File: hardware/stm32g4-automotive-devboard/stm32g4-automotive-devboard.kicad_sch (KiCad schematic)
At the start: 0 parts

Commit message: Added mcu and trancievers to sch
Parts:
- added U1: STM32G431CBTx, Package_QFP:LQFP-48_7x7mm_P0.5mm, symbol MCU_ST_STM32G4:STM32G431CBTx
- added U2, U3: TJA1051T-3, Package_SO:SOIC-8_3.9x4.9mm_P1.27mm, symbol Interface_CAN_LIN:TJA1051T-3
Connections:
- new net: U1.23 (VSS), U1.35 (VSS), U1.47 (VSS)

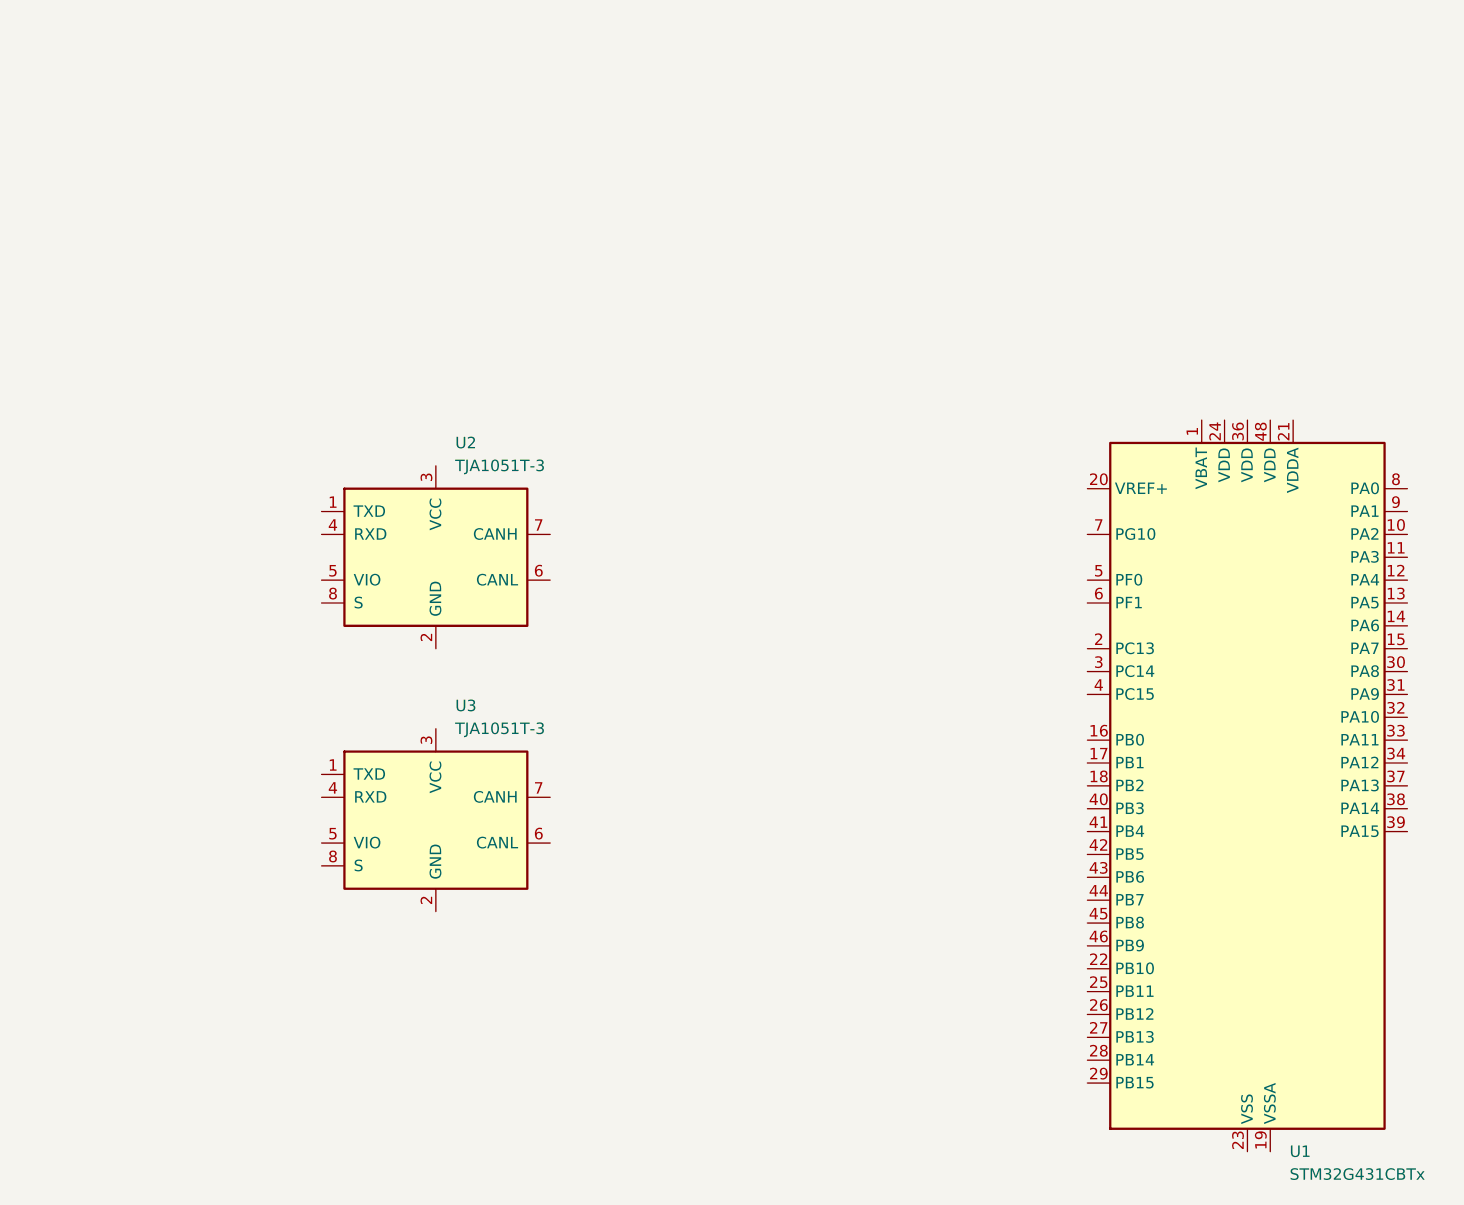
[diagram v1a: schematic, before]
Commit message: Updated Schematic and added bom.csv
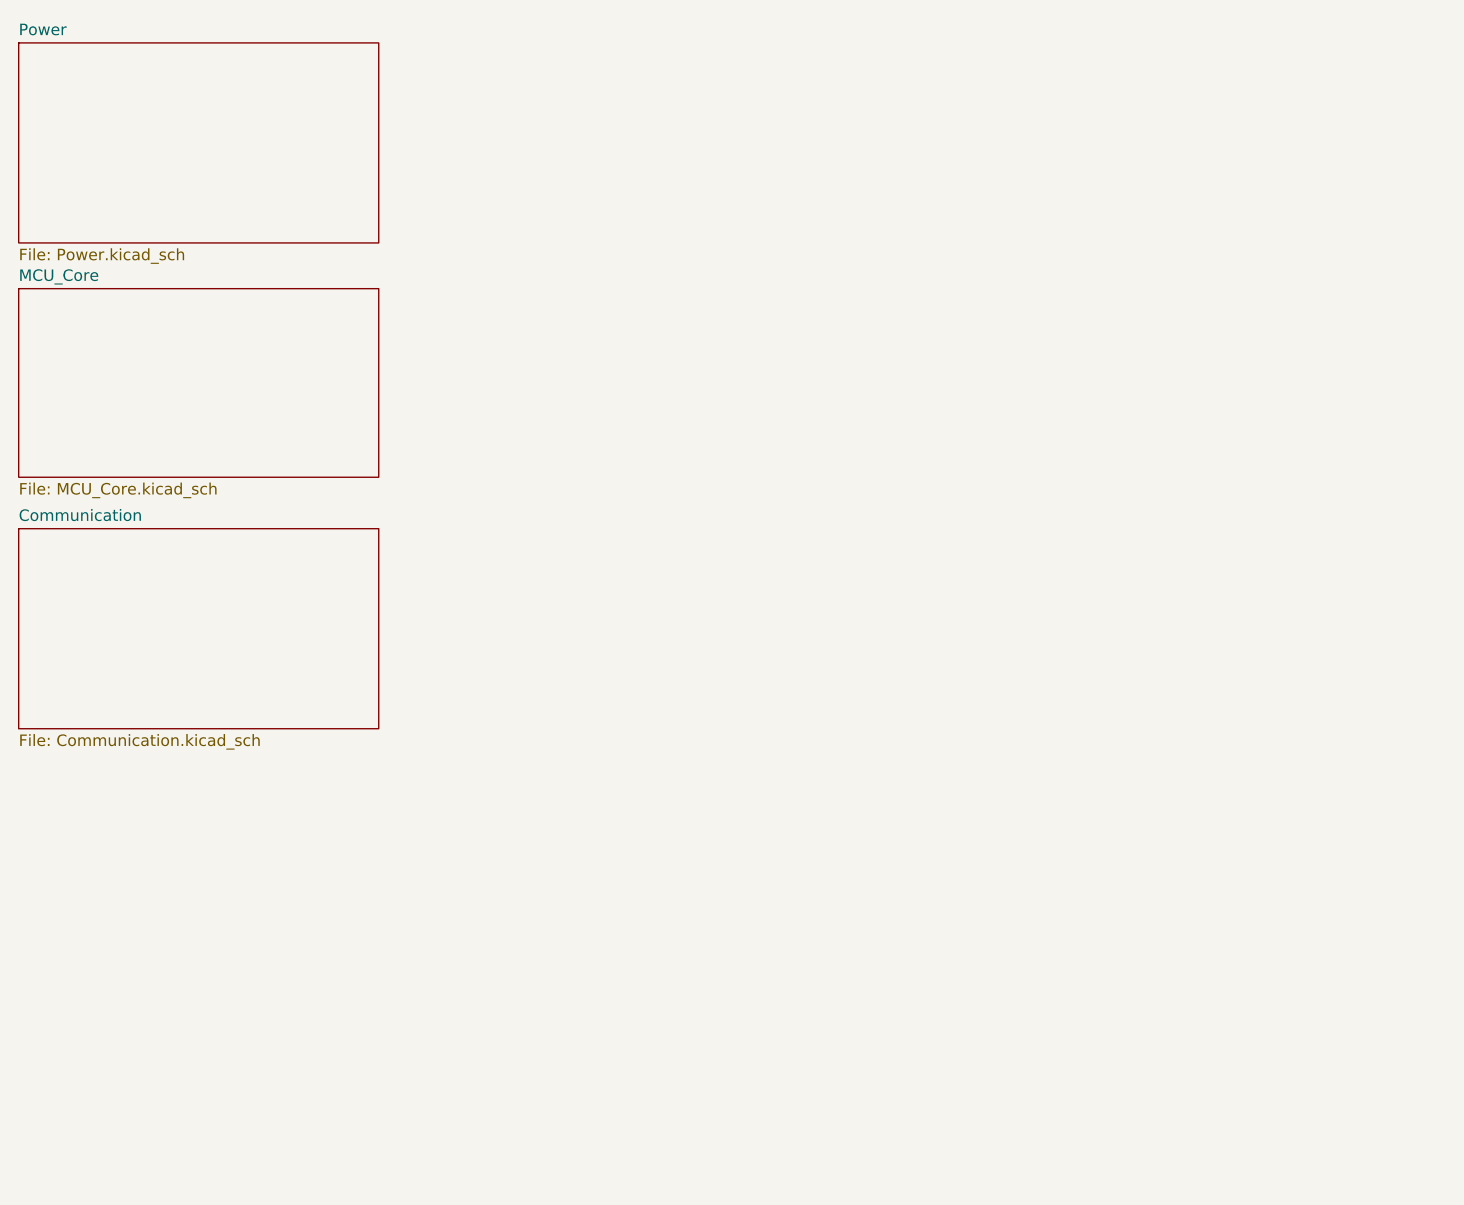
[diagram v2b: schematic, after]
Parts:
- removed U1: STM32G431CBTx, Package_QFP:LQFP-48_7x7mm_P0.5mm, symbol MCU_ST_STM32G4:STM32G431CBTx
- removed U2, U3: TJA1051T-3, Package_SO:SOIC-8_3.9x4.9mm_P1.27mm, symbol Interface_CAN_LIN:TJA1051T-3
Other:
- added sheet Communication (Communication.kicad_sch)
- added sheet MCU_Core (MCU_Core.kicad_sch)
- added sheet Power (Power.kicad_sch)
